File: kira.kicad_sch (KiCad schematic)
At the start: 35 parts, among them J1 USB_C_Receptacle_USB2.0, J2 SWD, SW37 SW_Push, SW46 Boot, SW47 Reset, U1 RP2040, U2 XC6206PxxxMR, U3 W25Q128JVS, U4 USBLC6-2SC6, Y1 12MHz

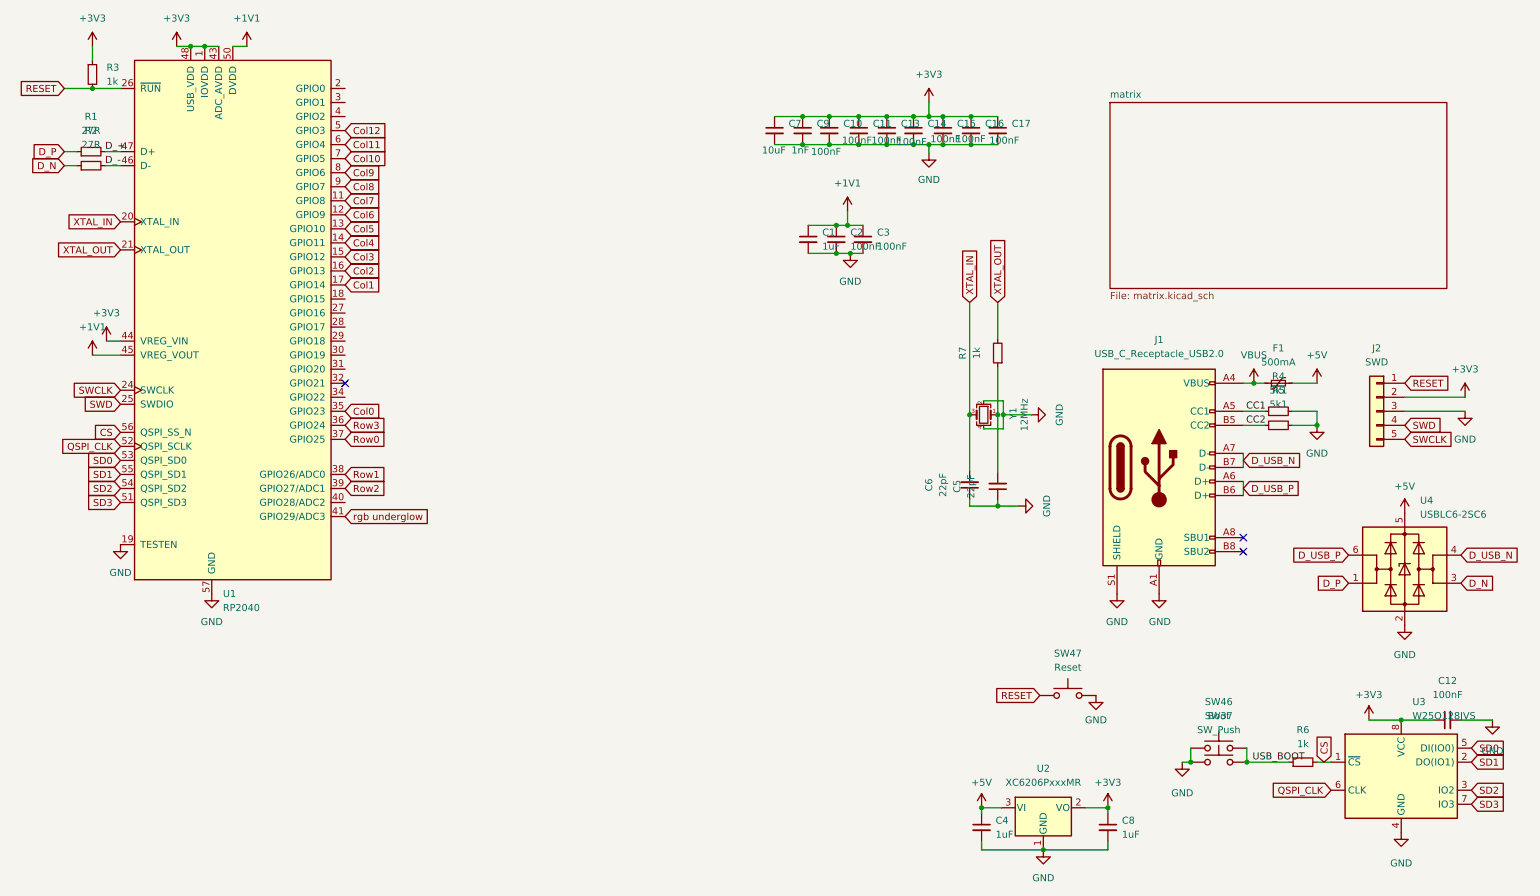
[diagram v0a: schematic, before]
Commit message: quick schematics cleanup
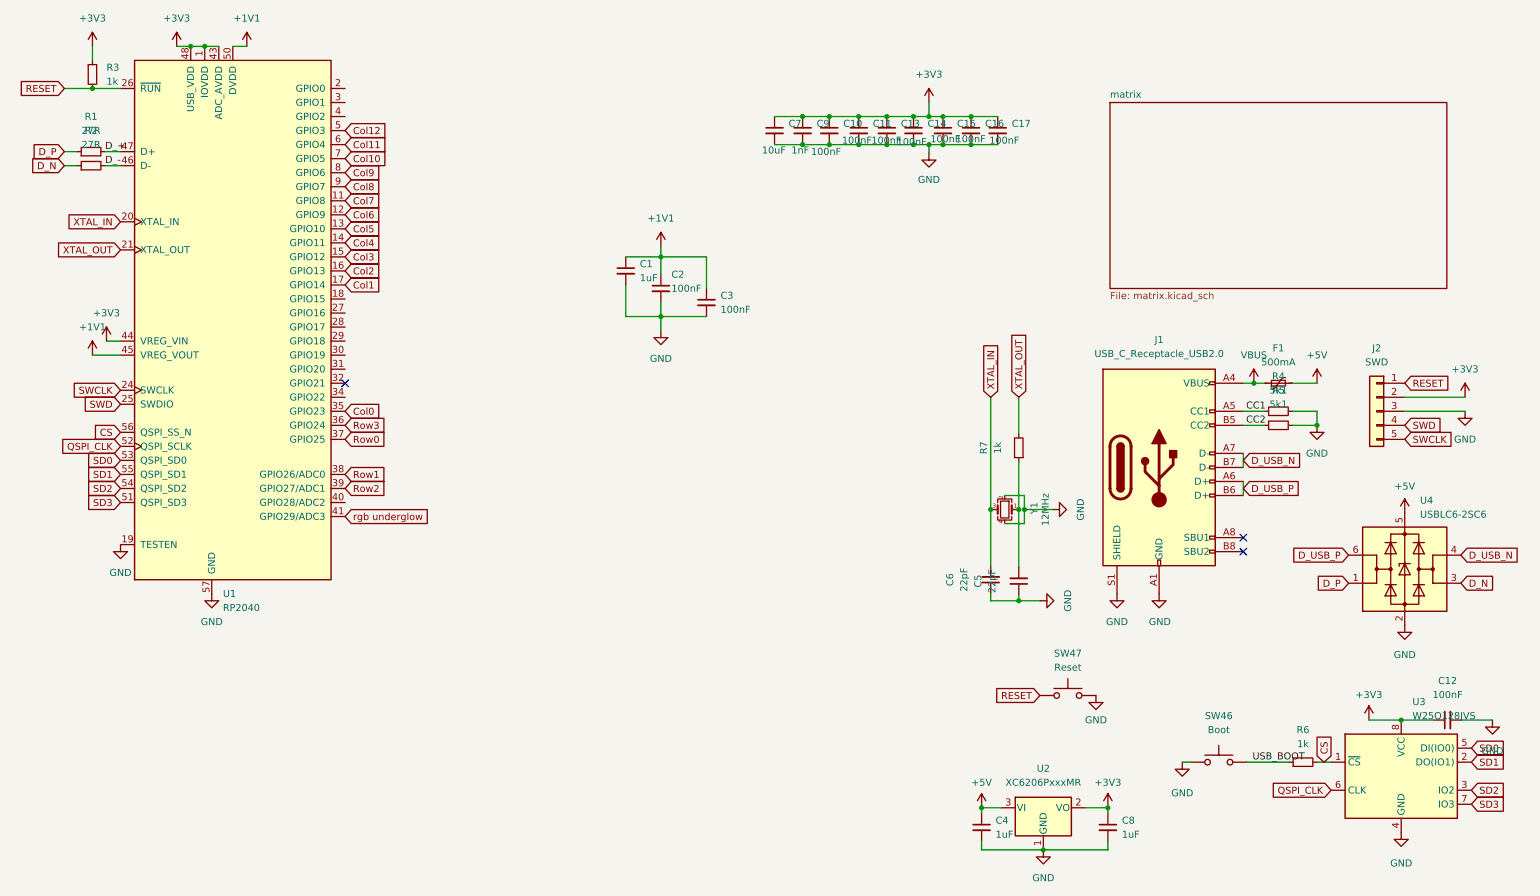
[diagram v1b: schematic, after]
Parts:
- removed SW37: SW_Push, Connector_PinHeader_2.00mm:PinHeader_1x02_P2.00mm_Vertical, symbol Switch:SW_Push
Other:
- moved on the sheet: C1, C2, C3, C5, C6, R7, SW46, Y1
